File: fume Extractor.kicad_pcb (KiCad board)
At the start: 2 copper layers, 49.8 x 32.2 mm, 13 parts, among them J1 FAN, Q1 BC337, SW1 SW_SPST, U1 L7805ACV

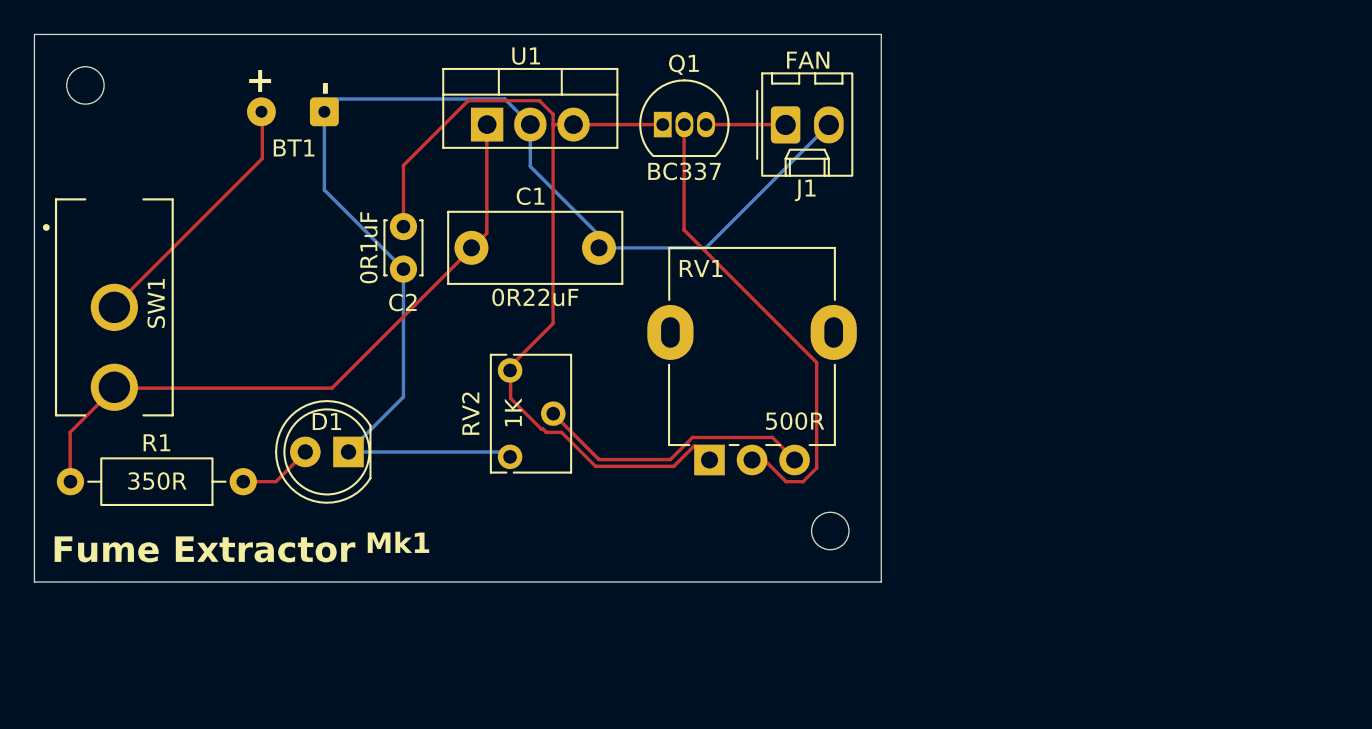
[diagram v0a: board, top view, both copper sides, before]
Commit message: Add Version 2
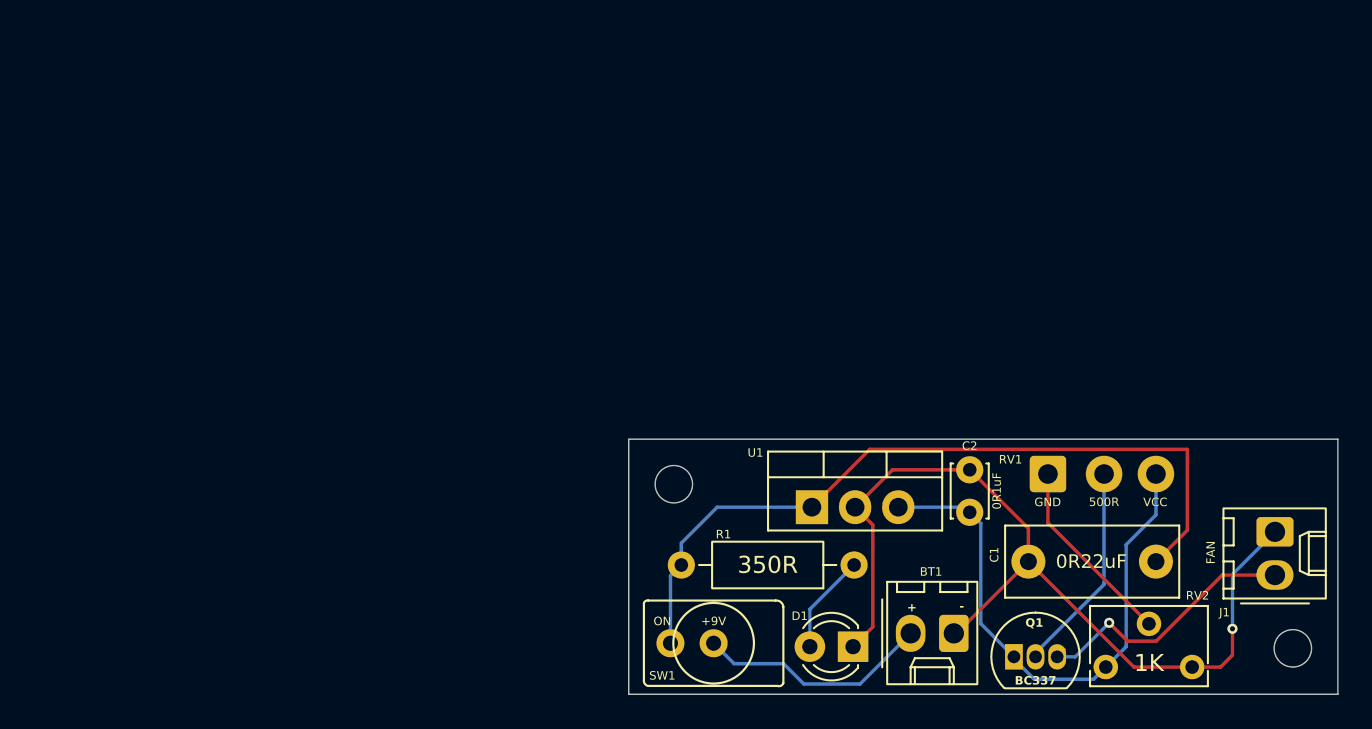
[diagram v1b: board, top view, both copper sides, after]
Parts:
- removed ?: MountingHole_2.2mm_M2, MountingHole:MountingHole_2.2mm_M2
- removed the REF** at (113.6, 83.4)
- added REF**: MountingHole_2.2mm_M2, MountingHole:MountingHole_2.2mm_M2, F.Cu at (104.4, 80.7)
- added REF**: MountingHole_2.2mm_M2, MountingHole:MountingHole_2.2mm_M2, F.Cu at (140.8, 90.3)
- BT1: footprint Connector_Wire:SolderWire-0.127sqmm_1x02_P3.7mm_D0.48mm_OD1mm -> Connector_Molex:Molex_KK-254_AE-6410-02A_1x02_P2.54mm_Vertical
- D1: value LED_5mm -> LED_3mm; footprint LED_THT:LED_D5.0mm -> LED_THT:LED_D3.0mm
- RV1: footprint Potentiometer_THT:Potentiometer_Alpha_RD901F-40-00D_Single_Vertical -> Connector_Wire:SolderWire-0.5sqmm_1x03_P4.6mm_D0.9mm_OD2.1mm
- SW1: footprint User_Passives:SW_SPDT_100SP1T1B4M2QE -> PCM_4ms_Switch:Switch_Toggle_SPDT_SubMini
- moved BT1 49.0 mm to (118.3, 89.4)
- moved C1 44.3 mm to (132.8, 85.2), turned to 180 degrees
- moved SW1 40.4 mm to (106.7, 90.0), turned to 90 degrees
- moved RV2 39.1 mm to (129.8, 91.4), turned to 180 degrees
- moved J1 39.1 mm to (139.8, 86.0), turned to 90 degrees
- moved Q1 37.5 mm to (124.4, 90.8)
- moved R1 36.3 mm to (115.0, 85.4)
- moved C2 35.3 mm to (121.8, 79.8), turned to -90 degrees
- moved D1 31.8 mm to (114.9, 90.2)
- moved U1 29.5 mm to (112.5, 82.0)
- moved RV1 18.6 mm to (125.1, 80.0), turned to 0 degrees
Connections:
- RV1 pad 1: Net-(Q1-C) -> Net-(RV1-Pad1)
- RV1 pad 3: Net-(RV1-Pad3) -> Net-(Q1-C)
- RV2 pad 2: Net-(RV1-Pad3) -> Net-(RV1-Pad1)
- SW1 pad 1: unconnected-(SW1-Pad1) -> Net-(U1-IN)
- SW1 pad 3: Net-(U1-IN) -> unconnected-(SW1-Pad3)
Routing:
- net Net-(Q1-C): track 52.4 -> 33.0 mm
- net -BATT: track 71.4 -> 52.9 mm, vias 0 -> 1
- net Net-(Q1-B): track 28.1 -> 11.6 mm
- net Net-(RV1-Pad3): track 16.4 -> 0.00 mm
- net Net-(J1-VCC): track 4.70 -> 16.3 mm, vias 0 -> 1
- net Net-(RV1-Pad1): track 0.00 -> 11.3 mm
- net Net-(U1-IN): track 38.6 -> 45.6 mm
- net Net-(D1-Pad2): track 4.30 -> 5.88 mm
- net +9V: track 15.0 -> 13.8 mm
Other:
- board size 49.8 x 32.2 mm -> 41.7 x 15 mm
- board text added: "+9V"
- board text added: "Fume Extractor^{ Mk2}"
- board text added: "GND"
- board text added: "ON"
- board text added: "VCC"
- board text removed: "Fume Extractor^{ Mk1}"
